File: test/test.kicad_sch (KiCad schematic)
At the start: 7 parts, among them J1 UEXT_Host

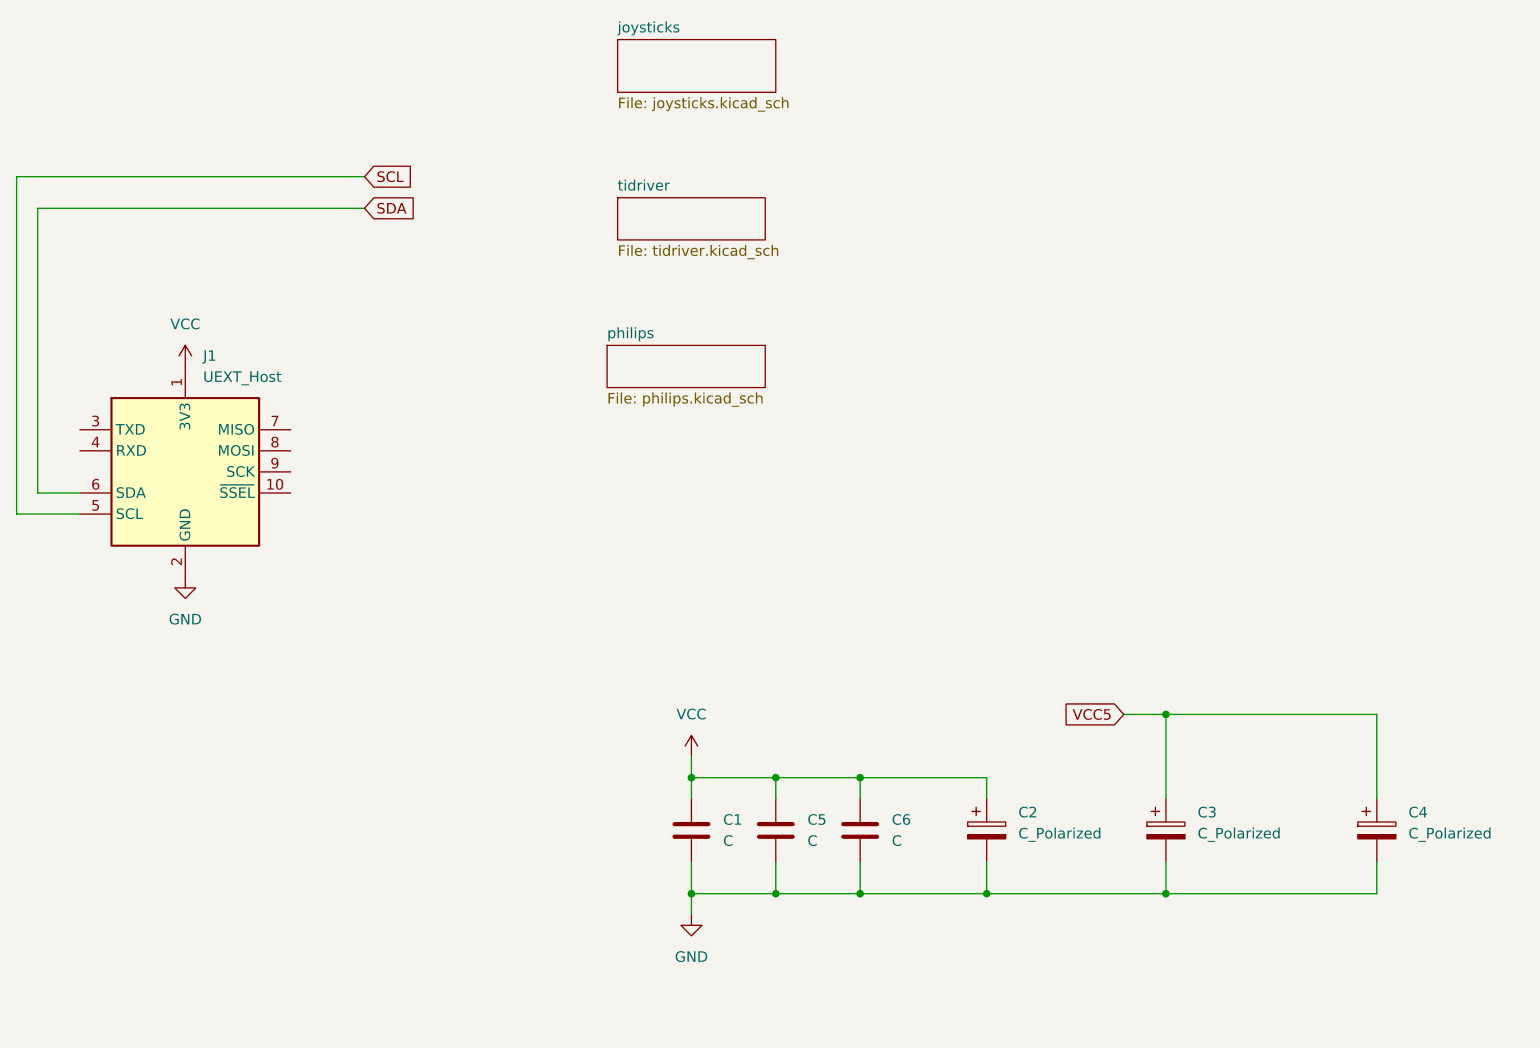
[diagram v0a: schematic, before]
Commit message: work on 2nd update test
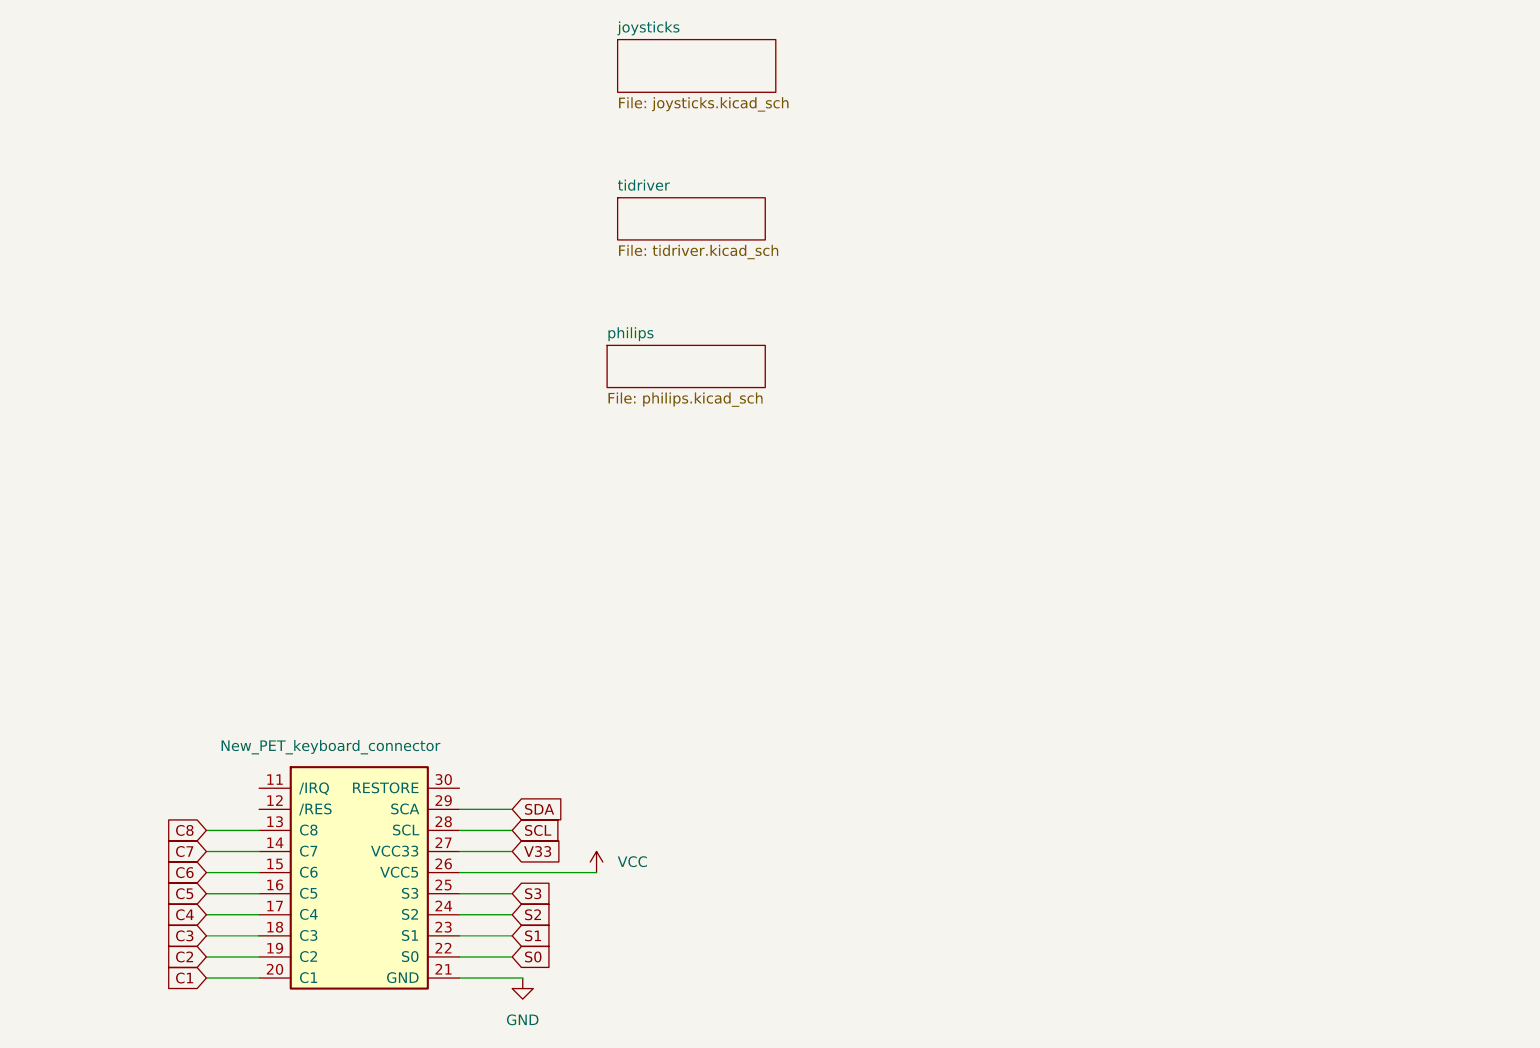
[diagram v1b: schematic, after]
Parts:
- removed C1, C5, C6: C, PCM_Diode_SMD_Handsoldering_AKL:D_0603_1608Metric, symbol Device:C
- removed C2, C3, C4: C_Polarized, Capacitor_THT:CP_Radial_D5.0mm_P2.00mm, symbol Device:C_Polarized
- removed J1: UEXT_Host, Connector_IDC:IDC-Header_2x05_P2.54mm_Vertical, symbol Connector:UEXT_Host
- added J6: New_PET_keyboard_connector, petkn:PET_New_Keyboard_Connector, symbol petkn:New_PET_keyboard_connector
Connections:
- net GND: now also J6.21 (GND)
- net SCL: now also J6.28 (SCL)
- net SDA: now also J6.29 (SCA)
- net VCC: now also J6.26 (VCC5)
- new net C1: J6.20 (C1)
- new net C2: J6.19 (C2)
- new net C3: J6.18 (C3)
- new net C4: J6.17 (C4)
- new net C5: J6.16 (C5)
- new net C6: J6.15 (C6)
- new net C7: J6.14 (C7)
- new net C8: J6.13 (C8)
- new net S0: J6.22 (S0)
- new net S1: J6.23 (S1)
- new net S2: J6.24 (S2)
- new net S3: J6.25 (S3)
- new net V33: J6.27 (VCC33)

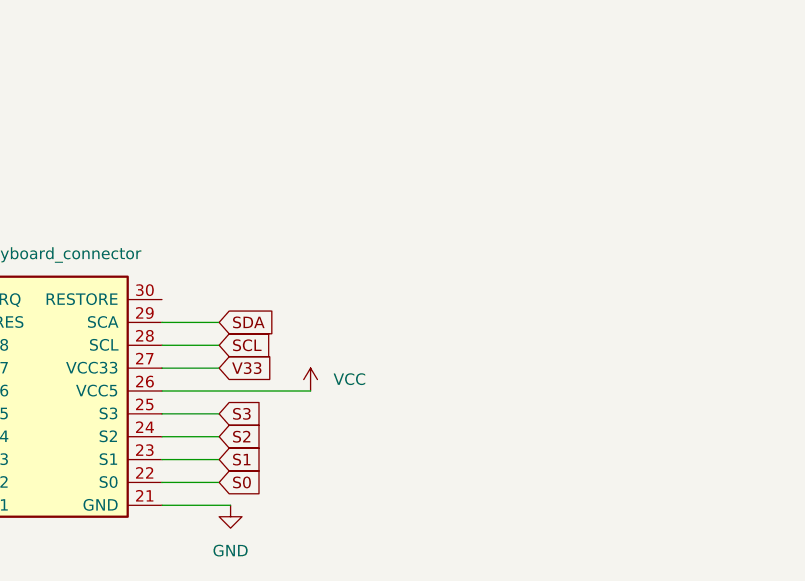
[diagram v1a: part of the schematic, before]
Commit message: production test pcb
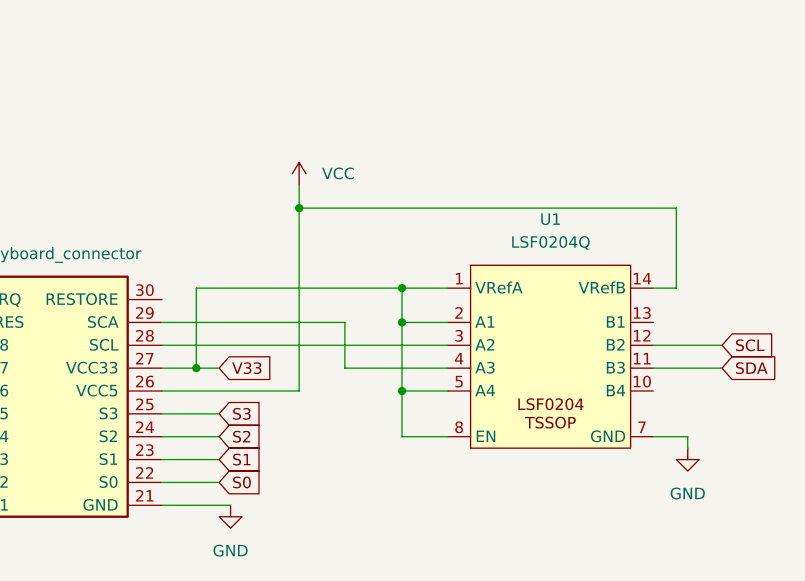
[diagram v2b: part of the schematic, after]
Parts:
- added U1: LSF0204Q, Package_SO:TSSOP-14_4.4x5mm_P0.65mm, symbol csa_petio_v1-eagle-import:LSF0204Q
- J6: LCSC (none) -> C492444
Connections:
- net GND: now also U1.7 (GND)
- net SCL: now also U1.12 (B2); no longer J6.28 (SCL)
- net SDA: now also U1.11 (B3); no longer J6.29 (SCA)
- net V33: now also U1.1 (VRefA), U1.2 (A1), U1.5 (A4), U1.8 (EN)
- net VCC: now also U1.14 (VRefB)
- new net: J6.28 (SCL), U1.3 (A2)
- new net: J6.29 (SCA), U1.4 (A3)
